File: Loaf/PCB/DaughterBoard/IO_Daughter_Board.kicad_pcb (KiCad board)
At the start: 2 copper layers, 100 x 72.8 mm, 18 parts, among them J1 DB25_Socket, J10 Ground Block 1, J11 5V Block, J12 Logic Block, J2 Barrel Jack, J7 Screw_Terminal_01x02, J8 Conn_01x02_Pin, J9 Ground Block 2, SW1 SW_Push

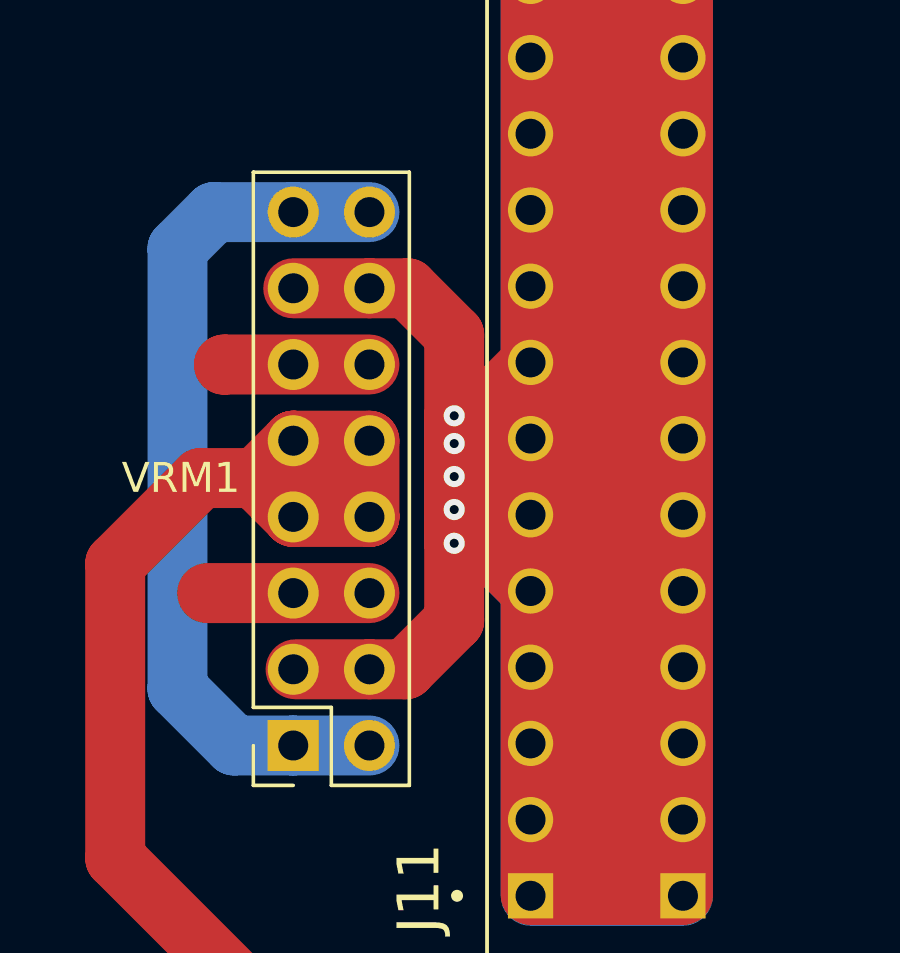
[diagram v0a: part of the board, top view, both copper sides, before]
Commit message: Added Gerbers
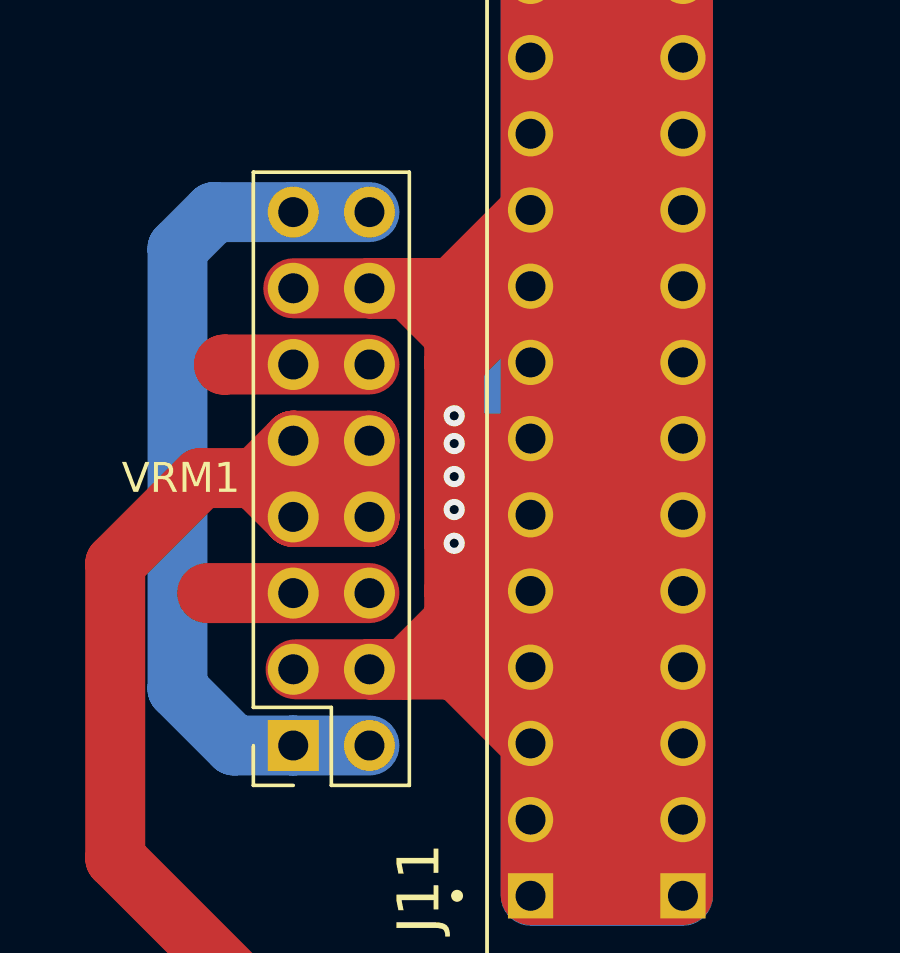
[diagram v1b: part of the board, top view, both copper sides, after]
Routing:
- net +5V: track 82.1 -> 113.0 mm
